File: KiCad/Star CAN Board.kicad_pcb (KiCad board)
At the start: 2 copper layers, 59.7 x 87.6 mm, 4 parts, among them J1 Conn_01x20_Female, J2 Conn_01x02_Male, J3 Conn_01x20_Female

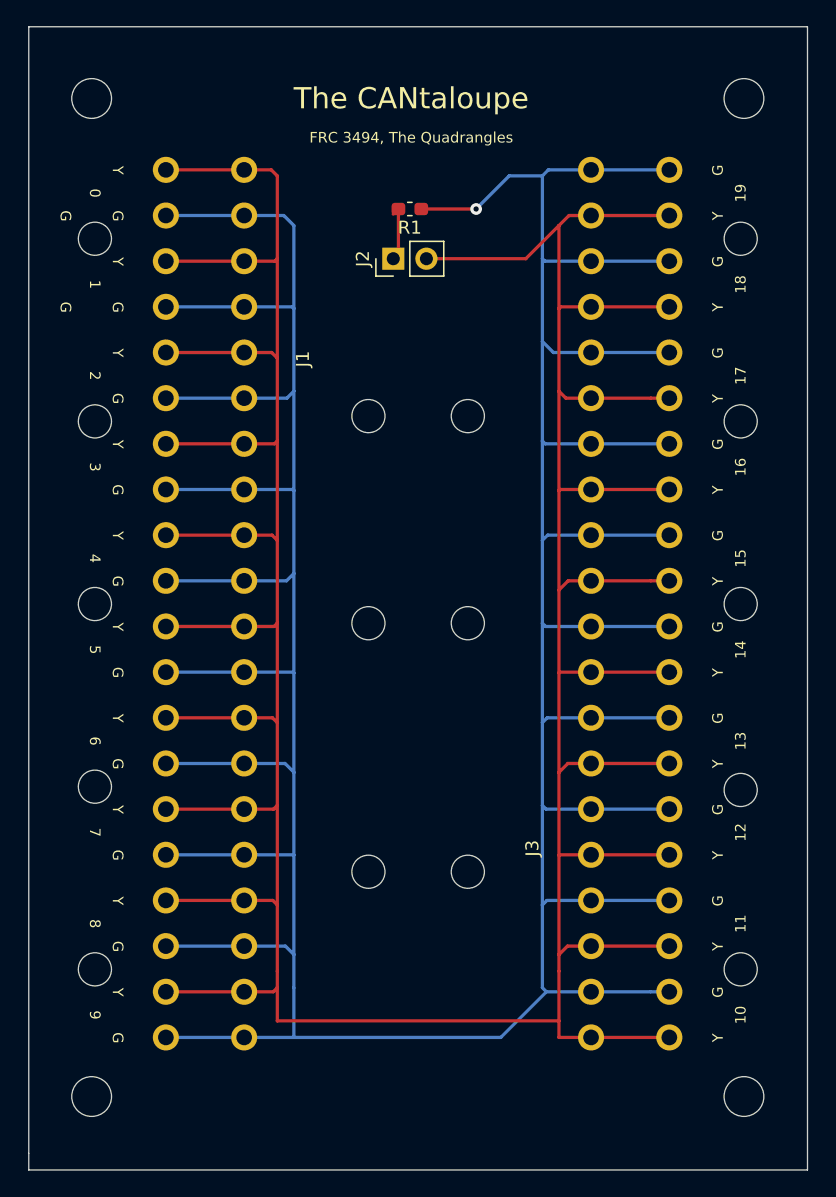
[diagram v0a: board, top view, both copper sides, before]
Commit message: hi this is FizzyApple12 pushing stuff for GraveFurball ok bye
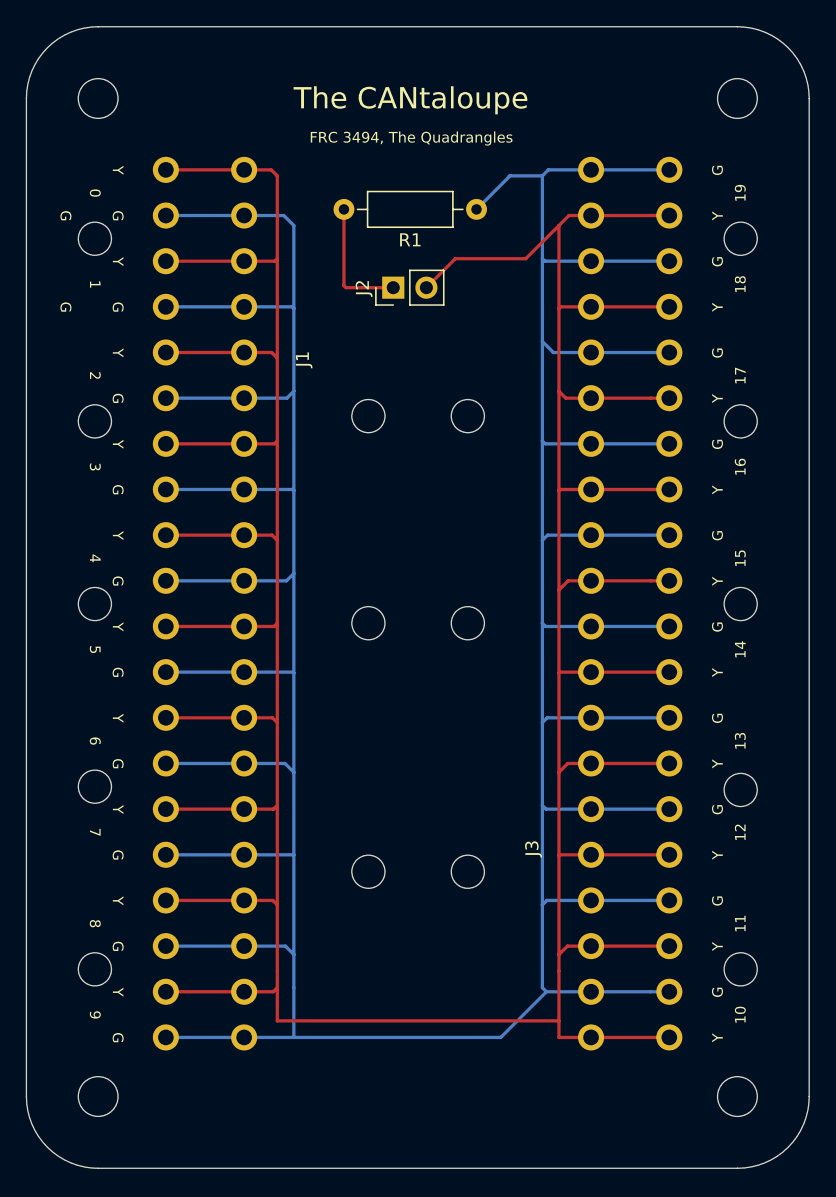
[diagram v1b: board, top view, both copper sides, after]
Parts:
- R1: footprint Resistor_SMD:R_0603_1608Metric_Pad1.05x0.95mm_HandSolder -> Resistor_THT:R_Axial_DIN0207_L6.3mm_D2.5mm_P10.16mm_Horizontal
- moved R1 5.11 mm to (141.0, 77.5)
- moved J2 2.22 mm to (134.6, 83.5)
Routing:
- net Net-(J2-Pad1): track 4.53 -> 9.69 mm
- net Net-(J1-Pad10): track 354.0 -> 349.8 mm, vias 1 -> 0
- net Net-(J1-Pad1): track 332.7 -> 333.6 mm
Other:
- board size 59.7 x 87.6 mm -> 60 x 87.5 mm
- board text added: "SCF 2020"
- board text added: "V1.1"
- board text removed: "SCF 2019"
- board text removed: "V1"
